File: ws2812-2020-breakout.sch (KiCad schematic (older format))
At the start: 6 parts, among them J1 Conn_01x02, J2 Conn_01x02

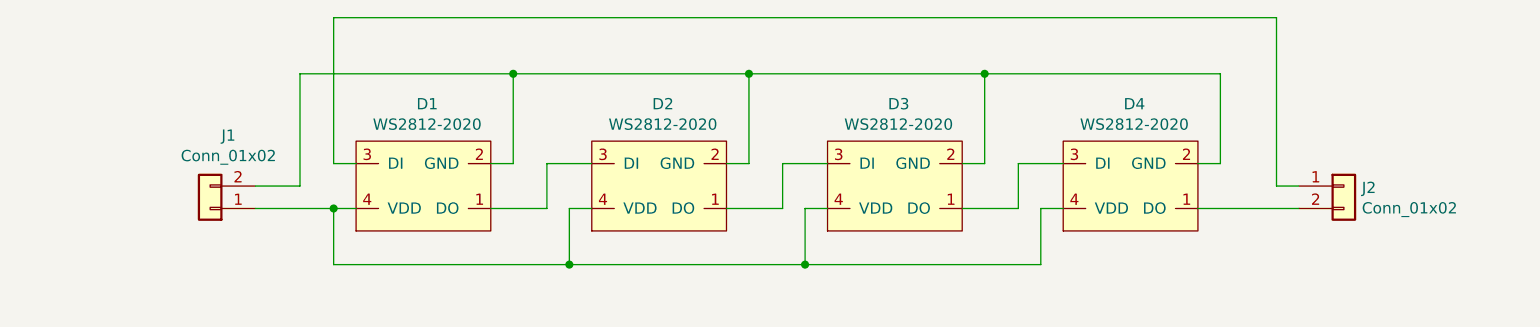
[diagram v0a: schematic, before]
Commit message: improve schematics
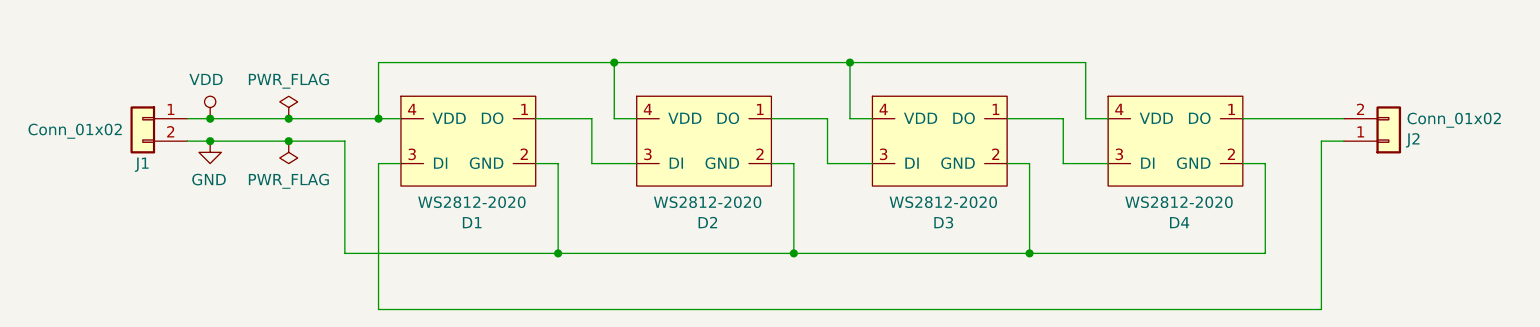
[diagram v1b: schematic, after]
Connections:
- net GND: now reaches D1.2 (GND), D2.2 (GND), D3.2 (GND), D4.2 (GND), J1.2 (Pin_2)
- net VDD: now reaches D1.4 (VDD), D2.4 (VDD), D3.4 (VDD), D4.4 (VDD), J1.1 (Pin_1)
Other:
- moved on the sheet: D1, D2, D3, D4, J1, J2
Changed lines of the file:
@@
 L LED:WS2812-2020 D1
 U 1 1 5DD38BD1
-P 4150 3950
-F 0 "D1" H 4167 4315 50  0000 C CNN
-F 1 "WS2812-2020" H 4167 4224 50  0000 C CNN
-F 2 "LED_SMD:WS2812-2020-2.00mmx2.20mm" H 4000 4150 50  0001 C CNN
-F 3 "http://www.peace-corp.co.jp/data/WS2812-2020_V1.0_EN.pdf" H 4000 4150 50  0001 C CNN
-	1    4150 3950
-	1    0    0    -1
+P 4350 3750
+F 0 "D1" H 4367 4115 50  0000 C CNN
+F 1 "WS2812-2020" H 4367 4024 50  0000 C CNN
+F 2 "LED_SMD:WS2812-2020-2.00mmx2.20mm" H 4200 3950 50  0001 C CNN
+F 3 "http://www.peace-corp.co.jp/data/WS2812-2020_V1.0_EN.pdf" H 4200 3950 50  0001 C CNN
+	1    4350 3750
+	1    0    0    1
 $EndComp
 $Comp
 L LED:WS2812-2020 D2
 U 1 1 5DD39655
-P 5200 3950
-F 0 "D2" H 5217 4315 50  0000 C CNN
-F 1 "WS2812-2020" H 5217 4224 50  0000 C CNN
-F 2 "LED_SMD:WS2812-2020-2.00mmx2.20mm" H 5050 4150 50  0001 C CNN
-F 3 "http://www.peace-corp.co.jp/data/WS2812-2020_V1.0_EN.pdf" H 5050 4150 50  0001 C CNN
-	1    5200 3950
-	1    0    0    -1
+P 5400 3750
+F 0 "D2" H 5417 4115 50  0000 C CNN
+F 1 "WS2812-2020" H 5417 4024 50  0000 C CNN
+F 2 "LED_SMD:WS2812-2020-2.00mmx2.20mm" H 5250 3950 50  0001 C CNN
+F 3 "http://www.peace-corp.co.jp/data/WS2812-2020_V1.0_EN.pdf" H 5250 3950 50  0001 C CNN
+	1    5400 3750
+	1    0    0    1
 $EndComp
 $Comp
 L LED:WS2812-2020 D3
 U 1 1 5DD3CD51
-P 6250 3950
-F 0 "D3" H 6267 4315 50  0000 C CNN
-F 1 "WS2812-2020" H 6267 4224 50  0000 C CNN
-F 2 "LED_SMD:WS2812-2020-2.00mmx2.20mm" H 6100 4150 50  0001 C CNN
-F 3 "http://www.peace-corp.co.jp/data/WS2812-2020_V1.0_EN.pdf" H 6100 4150 50  0001 C CNN
-	1    6250 3950
-	1    0    0    -1
-$EndComp
-Wire Wire Line
-	4550 3850 4450 3850
-Wire Wire Line
-	4450 4050 4700 4050
-Wire Wire Line
-	4700 4050 4700 3850
-Wire Wire Line
-	4700 3850 4900 3850
-Wire Wire Line
-	4800 4300 4800 4050
-Wire Wire Line
-	4800 4050 4900 4050
-Wire Wire Line
-	4800 4300 5850 4300
-Wire Wire Line
-	5850 4300 5850 4050
-Wire Wire Line
-	5850 4050 5950 4050
-Wire Wire Line
-	5850 4300 6900 4300
-Wire Wire Line
-	6900 4300 6900 4050
-Wire Wire Line
-	6900 4050 7000 4050
-Connection ~ 5850 4300
-Wire Wire Line
-	5500 4050 5750 4050
-Wire Wire Line
-	5750 4050 5750 3850
-Wire Wire Line
-	5750 3850 5950 3850
-Wire Wire Line
-	6550 4050 6800 4050
-Wire Wire Line
-	6800 4050 6800 3850
-Wire Wire Line
-	6800 3850 7000 3850
-Wire Wire Line
-	5600 3850 5500 3850
-Wire Wire Line
-	6650 3850 6550 3850
+P 6450 3750
+F 0 "D3" H 6467 4115 50  0000 C CNN
+F 1 "WS2812-2020" H 6467 4024 50  0000 C CNN
+F 2 "LED_SMD:WS2812-2020-2.00mmx2.20mm" H 6300 3950 50  0001 C CNN
+F 3 "http://www.peace-corp.co.jp/data/WS2812-2020_V1.0_EN.pdf" H 6300 3950 50  0001 C CNN
+	1    6450 3750
+	1    0    0    1
+$EndComp
+Wire Wire Line
+	4750 3850 4650 3850
+Wire Wire Line
+	4650 3650 4900 3650
+Wire Wire Line
+	4900 3650 4900 3850
+Wire Wire Line
+	4900 3850 5100 3850
+Wire Wire Line
+	5000 3400 5000 3650
+Wire Wire Line
+	5000 3650 5100 3650
+Wire Wire Line
+	5000 3400 6050 3400
+Wire Wire Line
+	6050 3400 6050 3650
+Wire Wire Line
+	6050 3650 6150 3650
+Wire Wire Line
+	6050 3400 7100 3400
+Wire Wire Line
+	7100 3400 7100 3650
+Wire Wire Line
+	7100 3650 7200 3650
+Connection ~ 6050 3400
+Wire Wire Line
+	5700 3650 5950 3650
+Wire Wire Line
+	5950 3650 5950 3850
+Wire Wire Line
+	5950 3850 6150 3850
+Wire Wire Line
+	6750 3650 7000 3650
+Wire Wire Line
+	7000 3650 7000 3850
+Wire Wire Line
+	7000 3850 7200 3850
+Wire Wire Line
+	5800 3850 5700 3850
+Wire Wire Line
+	6850 3850 6750 3850
 $Comp
 L Connector_Generic:Conn_01x02 J1
 U 1 1 5DD51DC0
-P 3200 4050
-F 0 "J1" H 3118 3725 50  0000 C CNN
-F 1 "Conn_01x02" H 3118 3816 50  0000 C CNN
-F 2 "Connector_PinSocket_2.54mm:PinSocket_1x02_P2.54mm_Vertical" H 3200 4050 50  0001 C CNN
-F 3 "~" H 3200 4050 50  0001 C CNN
-	1    3200 4050
-	-1   0    0    1
-$EndComp
-Wire Wire Line
-	3850 4050 3750 4050
-Wire Wire Line
-	4800 4300 3750 4300
-Wire Wire Line
-	3750 4300 3750 4050
-Connection ~ 4800 4300
-Connection ~ 3750 4050
-Wire Wire Line
-	3750 4050 3400 4050
+P 2900 3650
+F 0 "J1" H 2900 3450 50  0000 C CNN
+F 1 "Conn_01x02" H 3200 3600 50  0000 C CNN
+F 2 "Connector_PinSocket_2.54mm:PinSocket_1x02_P2.54mm_Vertical" H 2900 3650 50  0001 C CNN
+F 3 "~" H 2900 3650 50  0001 C CNN
+	1    2900 3650
+	-1   0    0    -1
+$EndComp
+Wire Wire Line
+	4050 3650 3950 3650
+Wire Wire Line
+	5000 3400 3950 3400
+Wire Wire Line
+	3950 3400 3950 3650
+Connection ~ 5000 3400
+Connection ~ 3950 3650
 $Comp
 L Connector_Generic:Conn_01x02 J2
 U 1 1 5DD5269B
-P 8250 3950
-F 0 "J2" H 8330 3942 50  0000 L CNN
-F 1 "Conn_01x02" H 8330 3851 50  0000 L CNN
-F 2 "Connector_PinSocket_2.54mm:PinSocket_1x02_P2.54mm_Vertical" H 8250 3950 50  0001 C CNN
-F 3 "~" H 8250 3950 50  0001 C CNN
-	1    8250 3950
-	1    0    0    -1
+P 8450 3750
+F 0 "J2" H 8530 3742 50  0000 L CNN
+F 1 "Conn_01x02" H 8530 3651 50  0000 L CNN
+F 2 "Connector_PinSocket_2.54mm:PinSocket_1x02_P2.54mm_Vertical" H 8450 3750 50  0001 C CNN
+F 3 "~" H 8450 3750 50  0001 C CNN
+	1    8450 3750
+	1    0    0    1
 $EndComp
 $Comp
 L LED:WS2812-2020 D4
 U 1 1 5DD3CD57
-P 7300 3950
-F 0 "D4" H 7317 4315 50  0000 C CNN
-F 1 "WS2812-2020" H 7317 4224 50  0000 C CNN
-F 2 "LED_SMD:WS2812-2020-2.00mmx2.20mm" H 7150 4150 50  0001 C CNN
-F 3 "http://www.peace-corp.co.jp/data/WS2812-2020_V1.0_EN.pdf" H 7150 4150 50  0001 C CNN
-	1    7300 3950
-	1    0    0    -1
-$EndComp
-Wire Wire Line
-	5600 3450 6650 3450
-Wire Wire Line
-	6650 3450 6650 3850
-Wire Wire Line
-	4550 3450 4550 3850
-Wire Wire Line
-	5600 3450 5600 3850
-Connection ~ 5600 3450
-Wire Wire Line
-	4550 3450 5600 3450
-Wire Wire Line
-	3850 3850 3750 3850
-Wire Wire Line
-	3750 3850 3750 3200
-Wire Wire Line
-	3750 3200 7950 3200
-Wire Wire Line
-	7950 3200 7950 3950
-Wire Wire Line
-	7950 3950 8050 3950
-Wire Wire Line
-	8050 4050 7600 4050
-Wire Wire Line
-	6650 3450 7700 3450
-Wire Wire Line
-	7700 3450 7700 3850
-Wire Wire Line
-	7700 3850 7600 3850
-Connection ~ 6650 3450
-Wire Wire Line
-	4550 3450 3600 3450
-Wire Wire Line
-	3600 3450 3600 3950
-Wire Wire Line
-	3600 3950 3400 3950
-Connection ~ 4550 3450
+P 7500 3750
+F 0 "D4" H 7517 4115 50  0000 C CNN
+F 1 "WS2812-2020" H 7517 4024 50  0000 C CNN
+F 2 "LED_SMD:WS2812-2020-2.00mmx2.20mm" H 7350 3950 50  0001 C CNN
+F 3 "http://www.peace-corp.co.jp/data/WS2812-2020_V1.0_EN.pdf" H 7350 3950 50  0001 C CNN
+	1    7500 3750
+	1    0    0    1
+$EndComp
+Wire Wire Line
+	5800 4250 6850 4250
+Wire Wire Line
+	6850 4250 6850 3850
+Wire Wire Line
+	4750 4250 4750 3850
+Wire Wire Line
+	5800 4250 5800 3850
+Connection ~ 5800 4250
+Wire Wire Line
+	4750 4250 5800 4250
+Wire Wire Line
+	4050 3850 3950 3850
+Wire Wire Line
+	3950 3850 3950 4500
+Wire Wire Line
+	3950 4500 8150 4500
+Wire Wire Line
+	8150 4500 8150 3750
+Wire Wire Line
+	8150 3750 8250 3750
+Wire Wire Line
+	8250 3650 7800 3650
+Wire Wire Line
+	6850 4250 7900 4250
+Wire Wire Line
+	7900 4250 7900 3850
+Wire Wire Line
+	7900 3850 7800 3850
+Connection ~ 6850 4250
+Wire Wire Line
+	4750 4250 3800 4250
+Wire Wire Line
+	3800 4250 3800 3750
+Connection ~ 4750 4250
+$Comp
+L power:PWR_FLAG #FLG0102
+U 1 1 5DCE801D
+P 3550 3750
+F 0 "#FLG0102" H 3550 3825 50  0001 C CNN
+F 1 "PWR_FLAG" H 3550 3923 50  0000 C CNN
+F 2 "" H 3550 3750 50  0001 C CNN
+F 3 "~" H 3550 3750 50  0001 C CNN
+	1    3550 3750
+	1    0    0    1
+$EndComp
+Connection ~ 3550 3750
+Wire Wire Line
+	3800 3750 3550 3750
+$Comp
+L power:PWR_FLAG #FLG0101
+U 1 1 5DCE39D7
+P 3550 3650
+F 0 "#FLG0101" H 3550 3725 50  0001 C CNN
+F 1 "PWR_FLAG" H 3550 3823 50  0000 C CNN
+F 2 "" H 3550 3650 50  0001 C CNN
+F 3 "~" H 3550 3650 50  0001 C CNN
+	1    3550 3650
+	-1   0    0    -1
+$EndComp
+Connection ~ 3550 3650
+Wire Wire Line
+	3950 3650 3550 3650
+$Comp
+L power:GND #PWR0101
+U 1 1 5DCED068
+P 3200 3750
+F 0 "#PWR0101" H 3200 3500 50  0001 C CNN
+F 1 "GND" H 3205 3577 50  0000 C CNN
+F 2 "" H 3200 3750 50  0001 C CNN
+F 3 "" H 3200 3750 50  0001 C CNN
+	1    3200 3750
+	-1   0    0    -1
+$EndComp
+Wire Wire Line
+	3550 3650 3200 3650
+Wire Wire Line
+	3550 3750 3200 3750
+Connection ~ 3200 3750
+Wire Wire Line
+	3200 3750 3100 3750
+$Comp
+L power:VDD #PWR0102
+U 1 1 5DCF1867
+P 3200 3650
+F 0 "#PWR0102" H 3200 3500 50  0001 C CNN
+F 1 "VDD" H 3217 3823 50  0000 C CNN
+F 2 "" H 3200 3650 50  0001 C CNN
+F 3 "" H 3200 3650 50  0001 C CNN
+	1    3200 3650
+	-1   0    0    -1
+$EndComp
+Connection ~ 3200 3650
+Wire Wire Line
+	3200 3650 3100 3650
 $EndSCHEMATC
